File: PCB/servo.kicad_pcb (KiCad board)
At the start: 4 copper layers, 24.5 x 45.9 mm, 24 parts, among them J1 Conn_ARM_SWD_TagConnect_TC203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, J2 Conn_01x04_MountingPin, J5 XKB-USB-C16PIN, U1 ATSAMD21E17D-M, U2 TMC6300-LA-T, U3 MA730, U4 LDK130PU33R_DFN6, U5 USBLC6-2P6

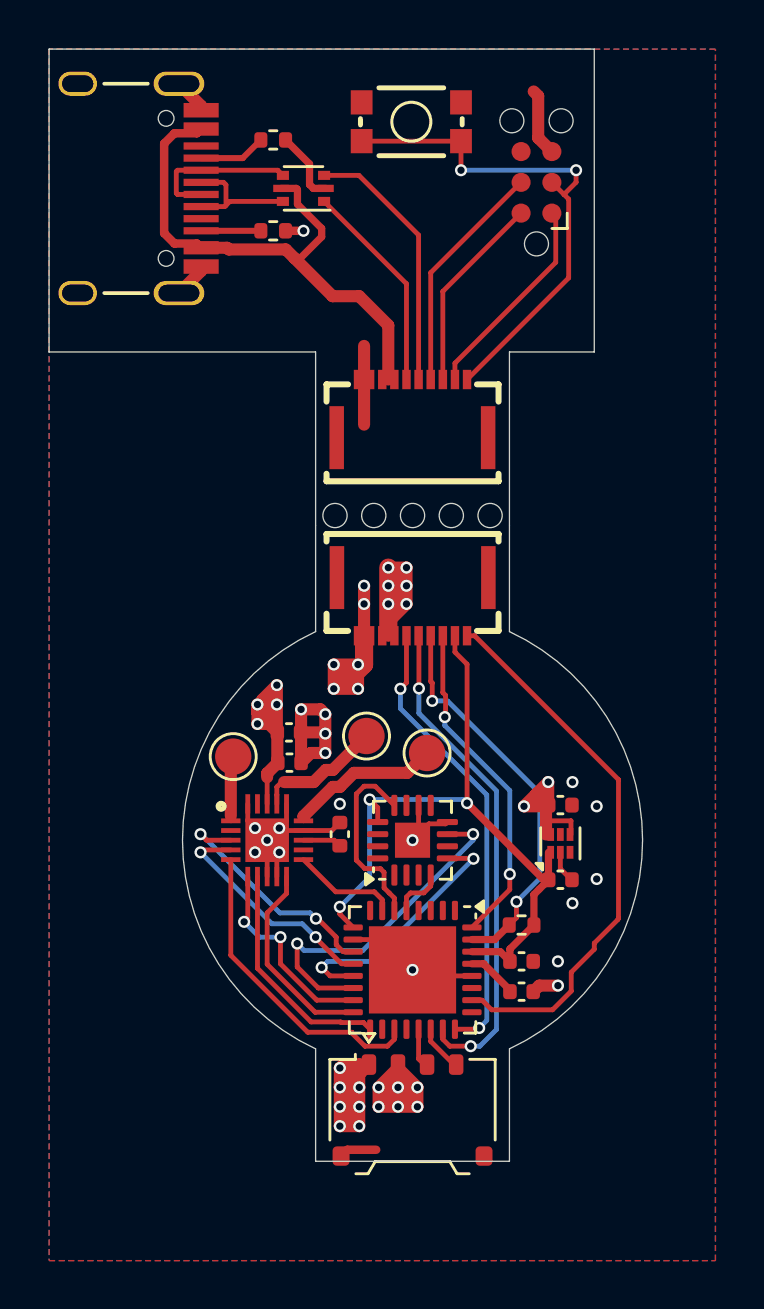
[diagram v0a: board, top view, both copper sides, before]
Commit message: Gerbers and changes
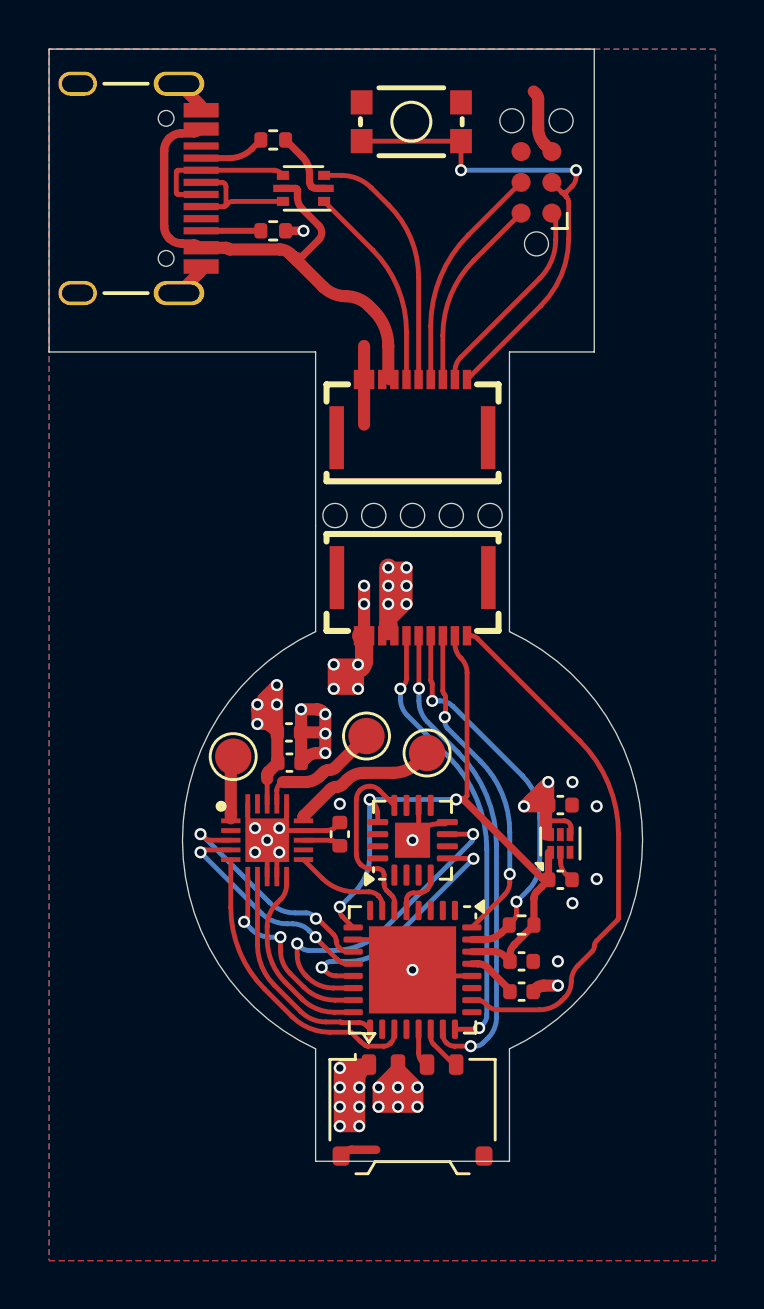
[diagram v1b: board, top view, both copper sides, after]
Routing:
- net +5V: track 66.7 -> 68.2 mm
- net D-: track 31.5 -> 30.8 mm
- net D+: track 27.7 -> 27.1 mm
- net SWCLK: track 26.2 -> 25.6 mm
- net +3.3V: track 38.5 -> 38.0 mm
